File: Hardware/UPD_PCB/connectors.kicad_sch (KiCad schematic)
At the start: 23 parts, among them J1 Screw_Terminal_01x02, J10 Screw_Terminal_01x02, J2 Conn_01x05_Pin, J3 Screw_Terminal_01x02, J4 Screw_Terminal_01x02, J5 Screw_Terminal_01x02, J6 Screw_Terminal_01x02, J7 Screw_Terminal_01x02, J8 Screw_Terminal_01x02, J9 Screw_Terminal_01x02

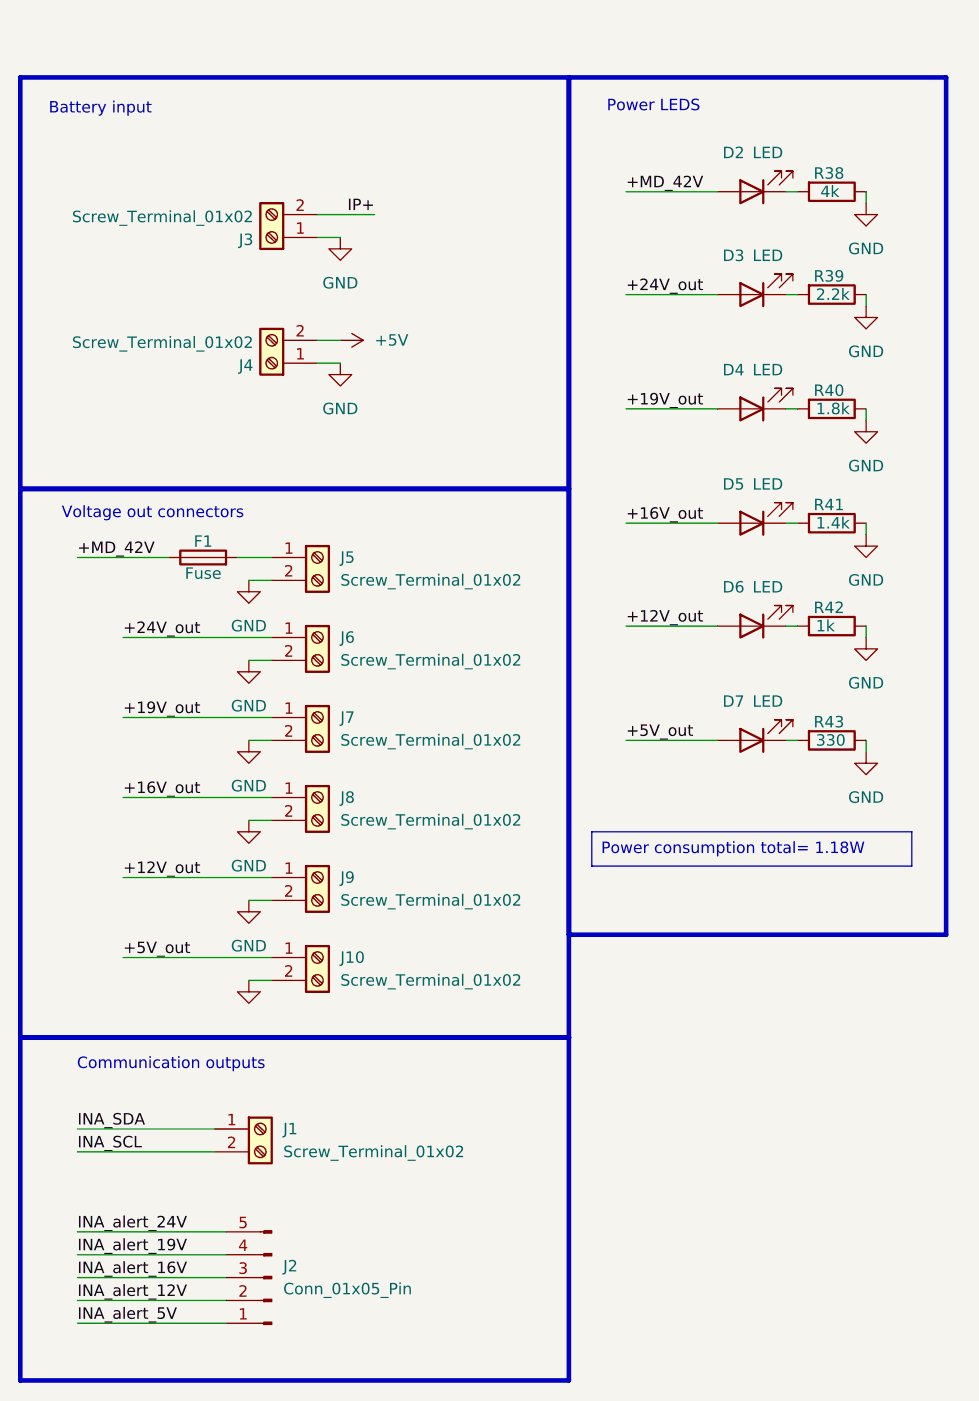
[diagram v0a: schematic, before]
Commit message: Finalized Schematic
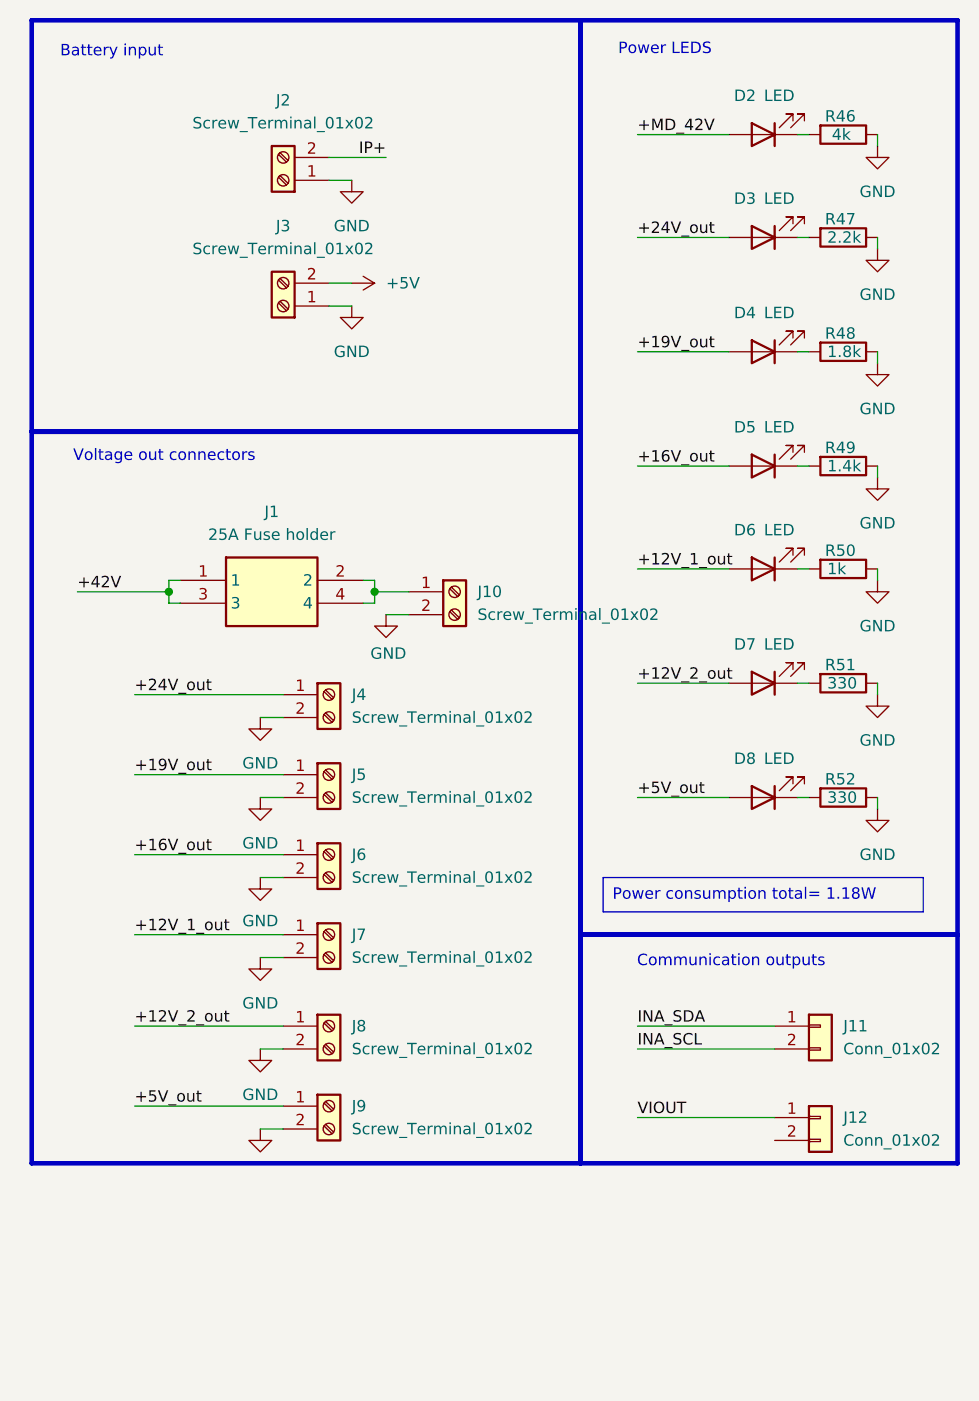
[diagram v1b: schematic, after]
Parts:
- removed F1: Fuse, symbol Device:Fuse
- removed J1: Screw_Terminal_01x02, symbol Connector:Screw_Terminal_01x02
- removed J2: Conn_01x05_Pin, Connector_PinHeader_1.00mm:PinHeader_1x05_P1.00mm_Vertical, symbol Connector:Conn_01x05_Pin
- added D8: LED, LED_SMD:LED_0603_1608Metric_Pad1.05x0.95mm_HandSolder, symbol Device:LED
- added J1: 25A Fuse holder, 3557-2, symbol 3557-2:3557-2
- added J11, J12: Conn_01x02, Connector_PinHeader_1.00mm:PinHeader_1x02_P1.00mm_Vertical, symbol Connector_Generic:Conn_01x02
- added J2: Screw_Terminal_01x02, TerminalBlock_Philmore:TerminalBlock_Philmore_TB132_1x02_P5.00mm_Horizontal, symbol Connector:Screw_Terminal_01x02
- added R52: 330, Resistor_SMD:R_0603_1608Metric_Pad0.98x0.95mm_HandSolder, symbol Device:R
- D5: footprint Resistor_SMD:R_0603_1608Metric_Pad0.98x0.95mm_HandSolder -> LED_SMD:LED_0603_1608Metric_Pad1.05x0.95mm_HandSolder
- J10, J3, J4, J5, J6, J7, J8, J9: footprint (none) -> TerminalBlock_Philmore:TerminalBlock_Philmore_TB132_1x02_P5.00mm_Horizontal
- renumbered R38 to R46, R39 to R47, R40 to R48, R41 to R49, R42 to R50, R43 to R51
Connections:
- net +16V_out: now also J6.1 (Pin_1); no longer J8.1 (Pin_1)
- net +19V_out: now also J5.1 (Pin_1); no longer J7.1 (Pin_1)
- net +24V_out: now also J4.1 (Pin_1); no longer J6.1 (Pin_1)
- net +5V: now also J3.2 (Pin_2); no longer J4.2 (Pin_2)
- net +5V_out: now also J9.1 (Pin_1), D8.2 (A); no longer D7.2 (A), J10.1 (Pin_1)
- net GND: now also J4.2 (Pin_2), J2.1 (Pin_1), R52.1; no longer J4.1 (Pin_1)
- net INA_SCL: now also J11.2 (Pin_2)
- net INA_SDA: now also J11.1 (Pin_1)
- net IP+: now also J2.2 (Pin_2); no longer J3.2 (Pin_2)
- net +12V_out renamed +12V_1_out
- net +12V_1_out: now also J7.1 (Pin_1); no longer J9.1 (Pin_1)
- new net: J1.2, J1.4, J10.1 (Pin_1)
- new net: D8.1 (K), R52.2
- new net +12V_2_out: D7.2 (A), J8.1 (Pin_1)
- new net +42V: J1.1, J1.3
- new net VIOUT: J12.1 (Pin_1)
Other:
- moved on the sheet: D2, D3, D4, D6, D7, R46, R47, R48, R49, R50, R51

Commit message: First board layout
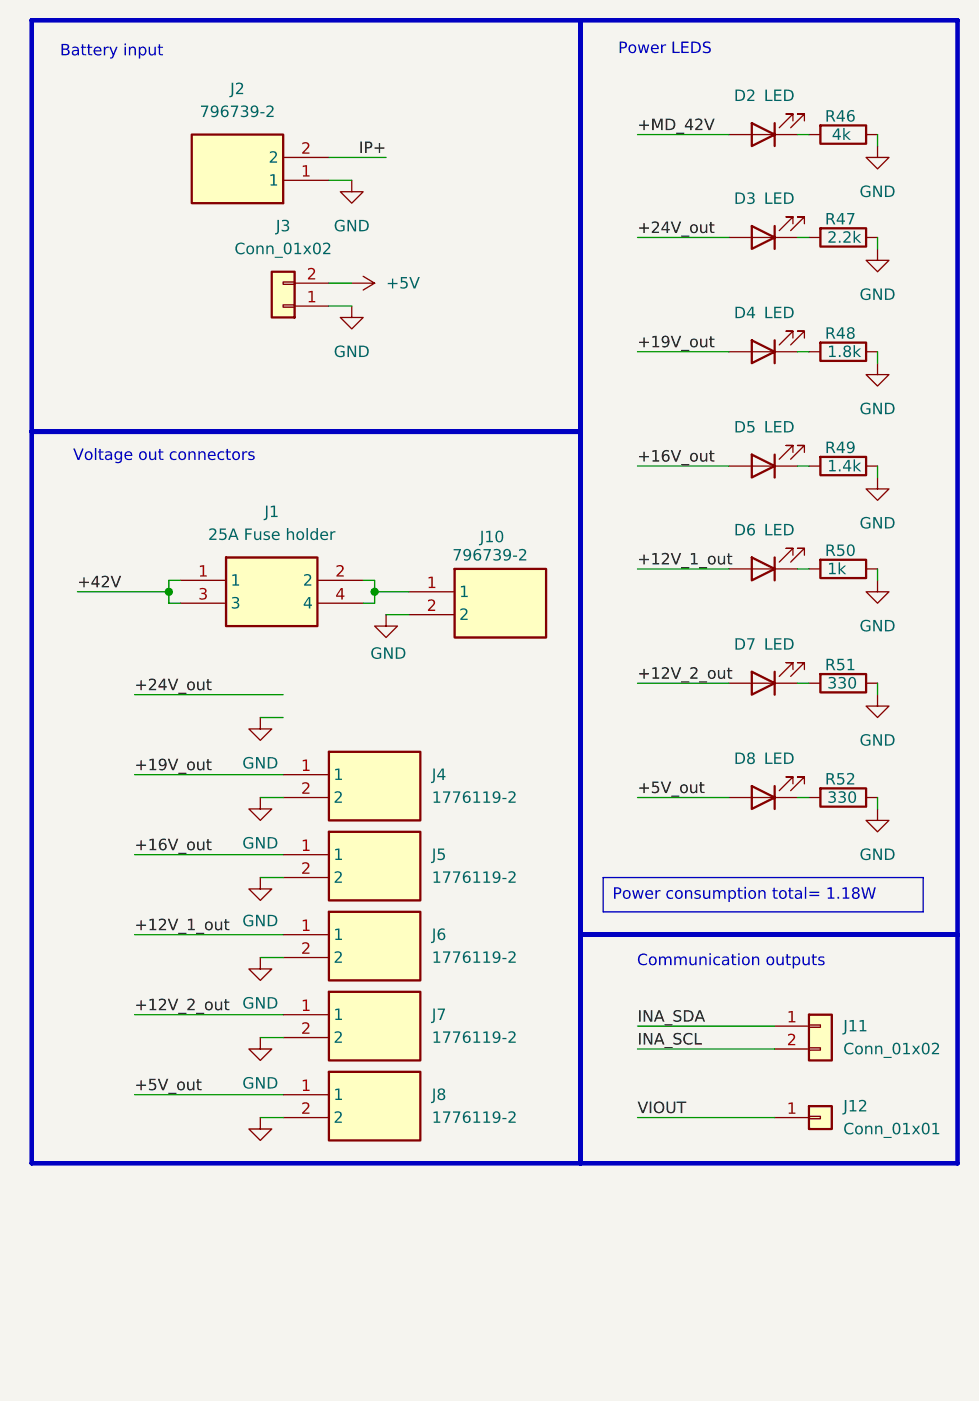
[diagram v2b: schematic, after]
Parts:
- removed J10, J2, J3, J4, J5, J6, J7, J8, J9: Screw_Terminal_01x02, TerminalBlock_Philmore:TerminalBlock_Philmore_TB132_1x02_P5.00mm_Horizontal, symbol Connector:Screw_Terminal_01x02
- removed J12: Conn_01x02, Connector_PinHeader_1.00mm:PinHeader_1x02_P1.00mm_Vertical, symbol Connector_Generic:Conn_01x02
- added J10, J2: 796739-2, 7967392, symbol 796739-2:796739-2
- added J12: Conn_01x01, Connector_PinHeader_1.00mm:PinHeader_1x01_P1.00mm_Vertical, symbol Connector_Generic:Conn_01x01
- added J3: Conn_01x02, Connector_PinHeader_1.00mm:PinHeader_1x02_P1.00mm_Vertical, symbol Connector_Generic:Conn_01x02
- added J4, J5, J6, J7, J8: 1776119-2, 17761192, symbol 1776119-2:1776119-2
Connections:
- net +12V_1_out: now also J6.1
- net +12V_2_out: now also J7.1
- net +16V_out: now also J5.1
- net +19V_out: now also J4.1
- net +5V: now also J3.2 (Pin_2)
- net +5V_out: now also J8.1
- net GND: now also J10.2, J2.1, J3.1 (Pin_1), J4.2, J5.2, J6.2, J7.2, J8.2
- net IP+: now also J2.2
- net VIOUT: now also J12.1 (Pin_1)
- net at J1.2, J1.4: now also J10.1
